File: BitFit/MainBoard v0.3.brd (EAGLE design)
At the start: 32.5 x 10.5 mm, 26 parts, among them J1 MICROUSB, U1 ATMEGA32U2QFN, U2 MCP738312, U3 LIS331, U5 REGULATOR

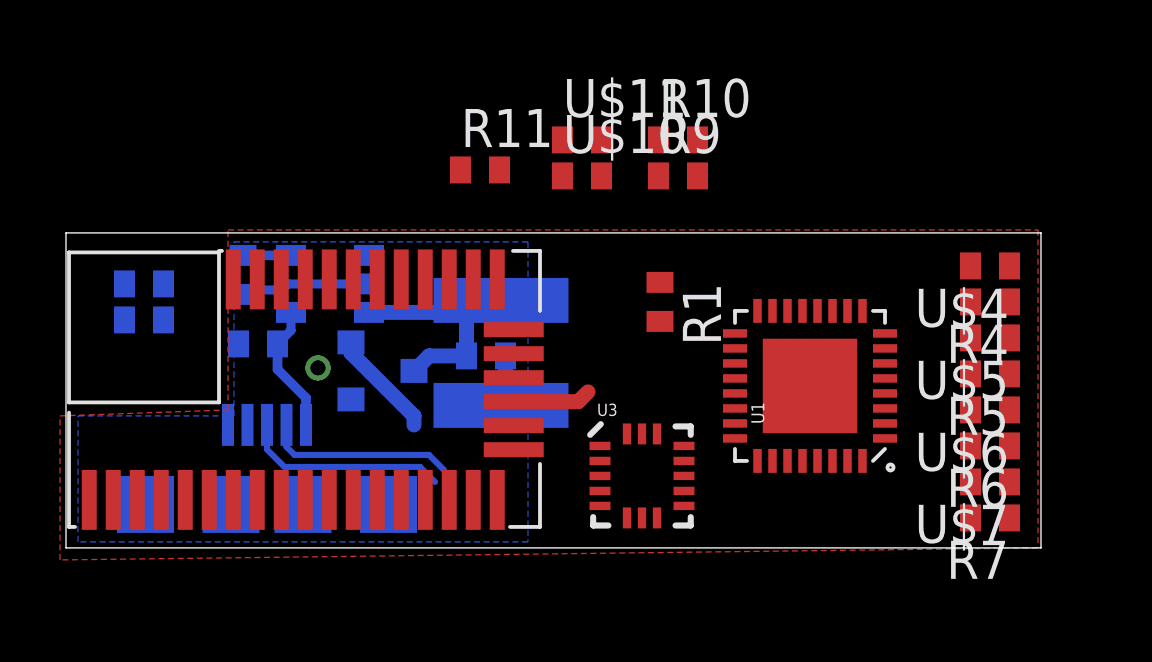
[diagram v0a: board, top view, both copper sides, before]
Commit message: Version 1.0
Finished version 1.0 of layout.
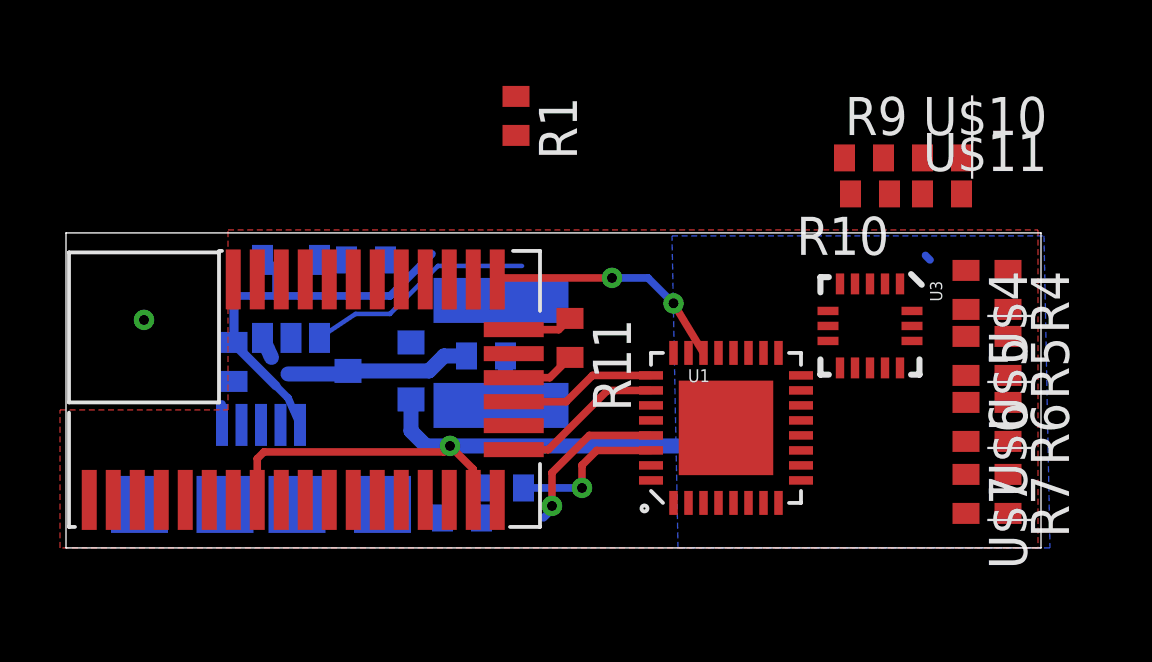
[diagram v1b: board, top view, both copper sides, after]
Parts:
- moved R2 13.2 mm to (14.6, 2.00)
- moved R3 13.2 mm to (13.2, 1.00)
- moved U$11 12.1 mm to (29.2, 11.8)
- moved U$10 12.0 mm to (29.2, 13.0)
- moved U3 9.10 mm to (26.8, 7.40), turned to 270 degrees
- moved R1 7.84 mm to (15.0, 14.4)
- moved R10 6.65 mm to (26.8, 11.8), turned to 180 degrees
- moved R11 6.35 mm to (16.8, 7.00), turned to 270 degrees
- moved R9 6.23 mm to (26.6, 13.0)
- moved R8 4.13 mm to (10.0, 9.60), turned to 180 degrees
- moved U1 3.13 mm to (22.0, 4.00), turned to 0 degrees
- moved U2 1.39 mm to (7.50, 8.30), turned to 0 degrees
- moved U$4 1.13 mm to (30.0, 8.60), turned to 270 degrees
- moved C2 1.00 mm to (5.60, 6.20), turned to 270 degrees
- moved U$5 1.00 mm to (30.0, 6.40), turned to 270 degrees
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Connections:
- net N$16: no longer A1.P$31
- net N$17: no longer A1.P$30
- net N$20: no longer A1.P$33
- net N$25: now also A1.P$31, U1.26; no longer U$7.2, U1.22
- net N$26: now also A1.P$30, U1.22; no longer U$6.2, U1.23
- net N$27: now also A1.P$33; no longer U$5.2
- net N$28: now also U1.1, U1.27; no longer U$4.2, U1.26
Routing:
- net +3V3: track 3.62 -> 21.1 mm, vias 0 -> 1
- net +5V: track 4.49 -> 13.7 mm
- net N$26: track 0.00 -> 8.18 mm, vias 0 -> 2
- net N$13: track 0.00 -> 7.87 mm
- net N$8: track 6.87 -> 0.21 mm
- net N$9: track 6.30 -> 0.00 mm
- net N$1: track 0.00 -> 5.44 mm, vias 0 -> 1
- net N$25: track 0.00 -> 5.39 mm
- net N$2: track 0.00 -> 5.21 mm, vias 0 -> 1
- net N$27: track 0.00 -> 4.94 mm
- net N$20: track 2.61 -> 0.00 mm
- net N$11: track 0.00 -> 2.15 mm
- net N$12: track 1.60 -> 0.00 mm
- net GND: track 6.51 -> 4.93 mm, vias 1 -> 0
- net N$10: track 9.49 -> 8.33 mm
- added copper zone on layer 16, net +3V3
- removed copper zone on layer 16, net GND
